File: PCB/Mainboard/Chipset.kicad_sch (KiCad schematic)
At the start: 19 parts, among them J4 connector-4, U19 74W126, U61 VL82C420FC5, U7 HD151015

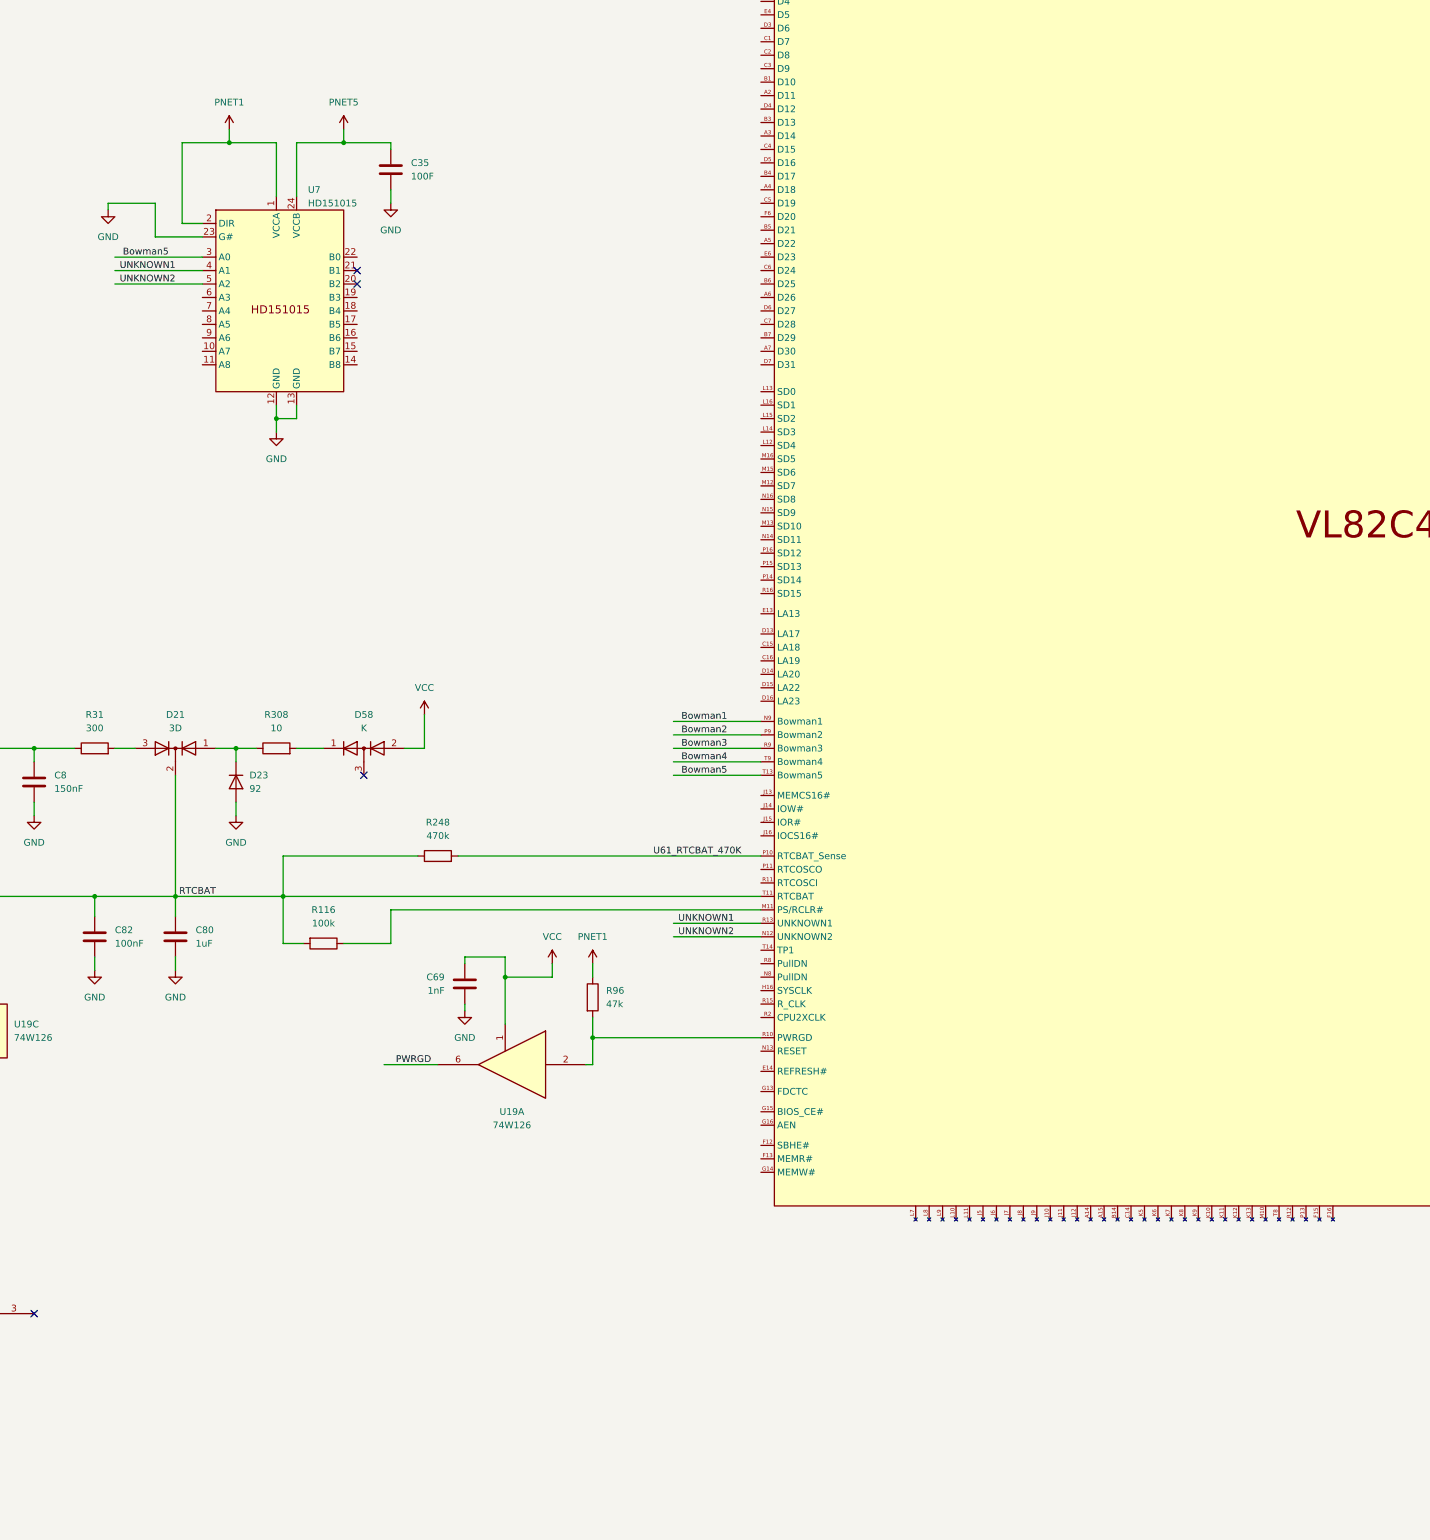
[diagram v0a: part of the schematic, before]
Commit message: Add files via upload
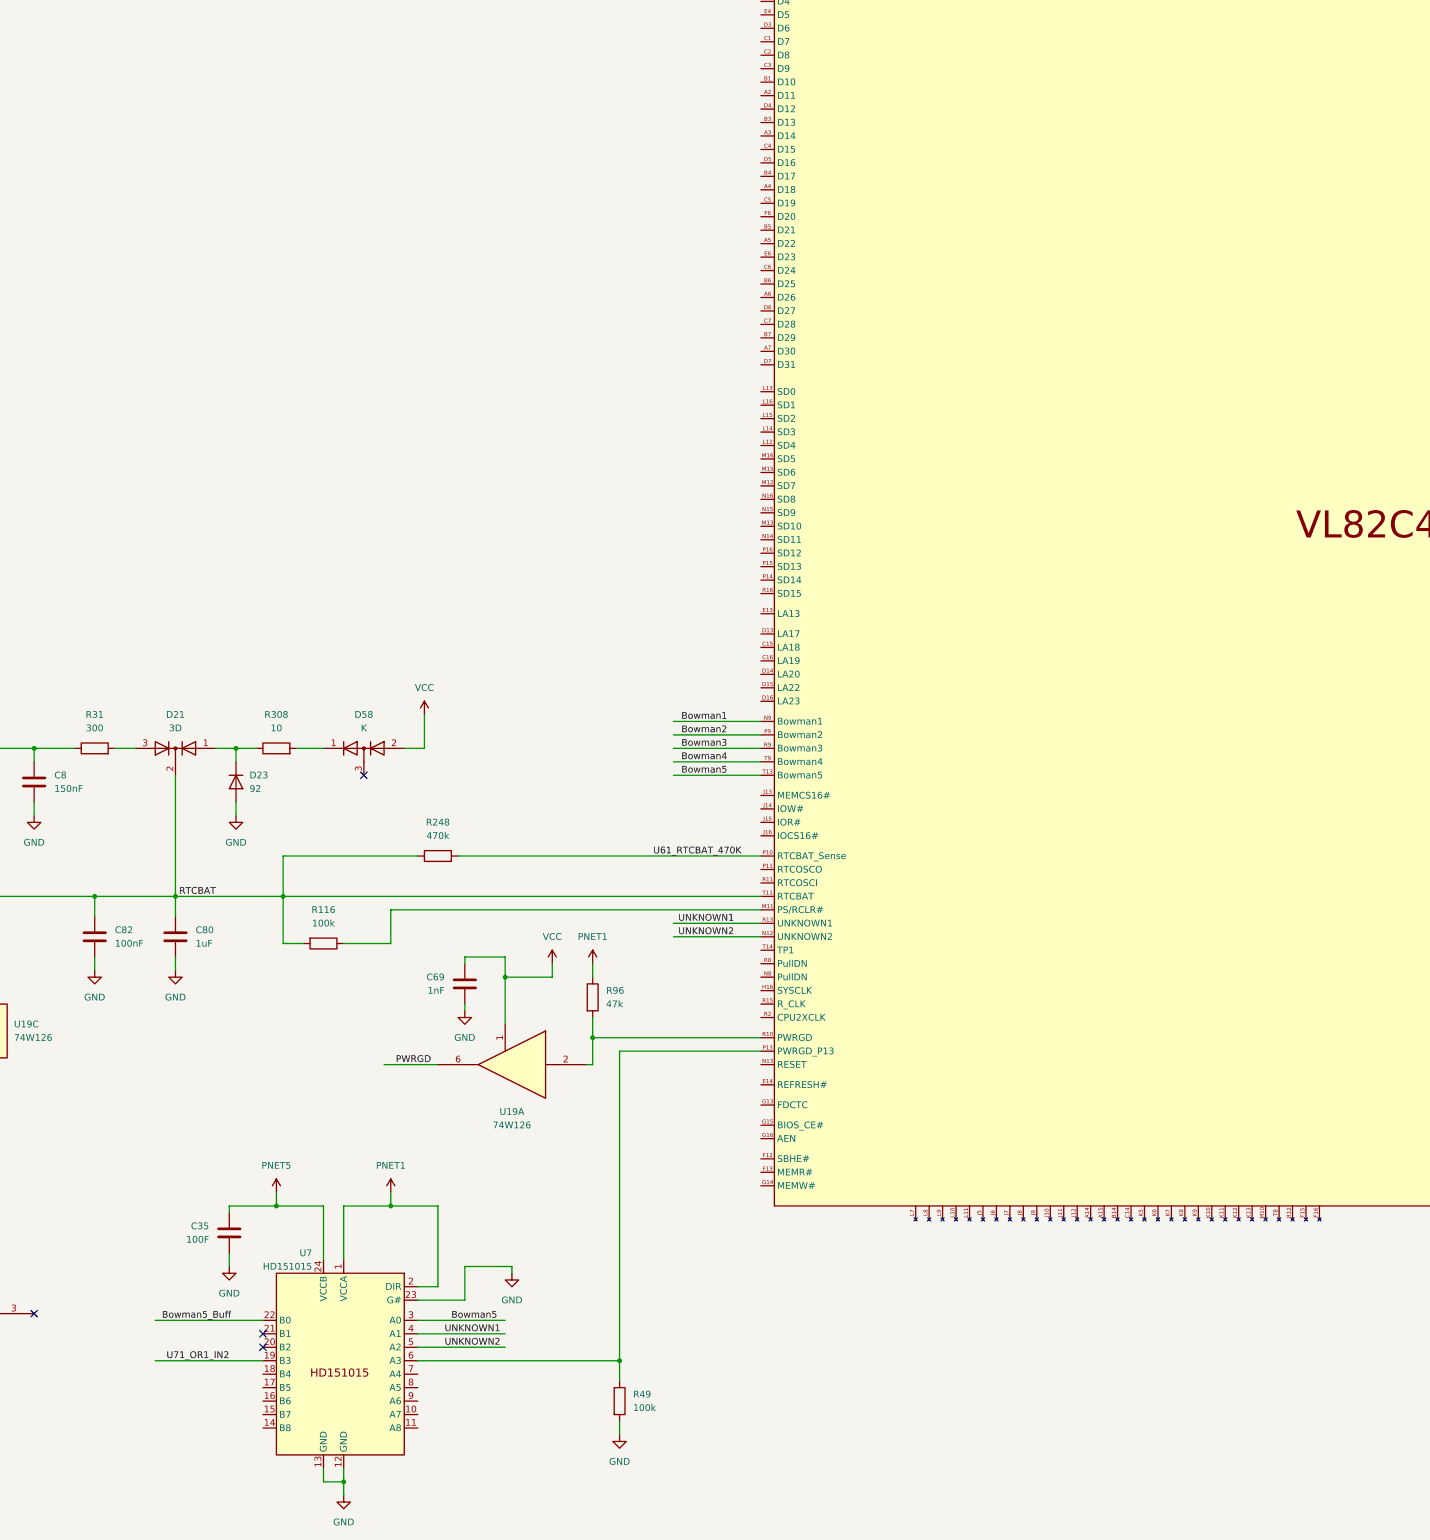
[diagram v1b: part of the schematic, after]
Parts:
- added R49: 100k, symbol Device:R
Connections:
- net GND: now also R49.2
- net at U61.P13 (PWRGD_P13): now also U7.6 (A3), R49.1
- net U71_OR1_IN2: now reaches U7.19 (B3)
- net Bowman5_Buff: now reaches U7.22 (B0)
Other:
- moved on the sheet: C35, U7
